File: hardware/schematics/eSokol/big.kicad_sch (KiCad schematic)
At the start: 34 parts, among them J6 BIGBATT_CHRG, M1 MY1016Z2, M2 FAN1, Q10 AO3401A, Q11 BC547, Q12 S8550, Q13 BC547, Q14 S8550, Q4 BC547, SW2 SW_MEASURE, SW8 SW_KEY, U10 LB27, U11 DS_VC288, U7 49e, U8 DS18S20

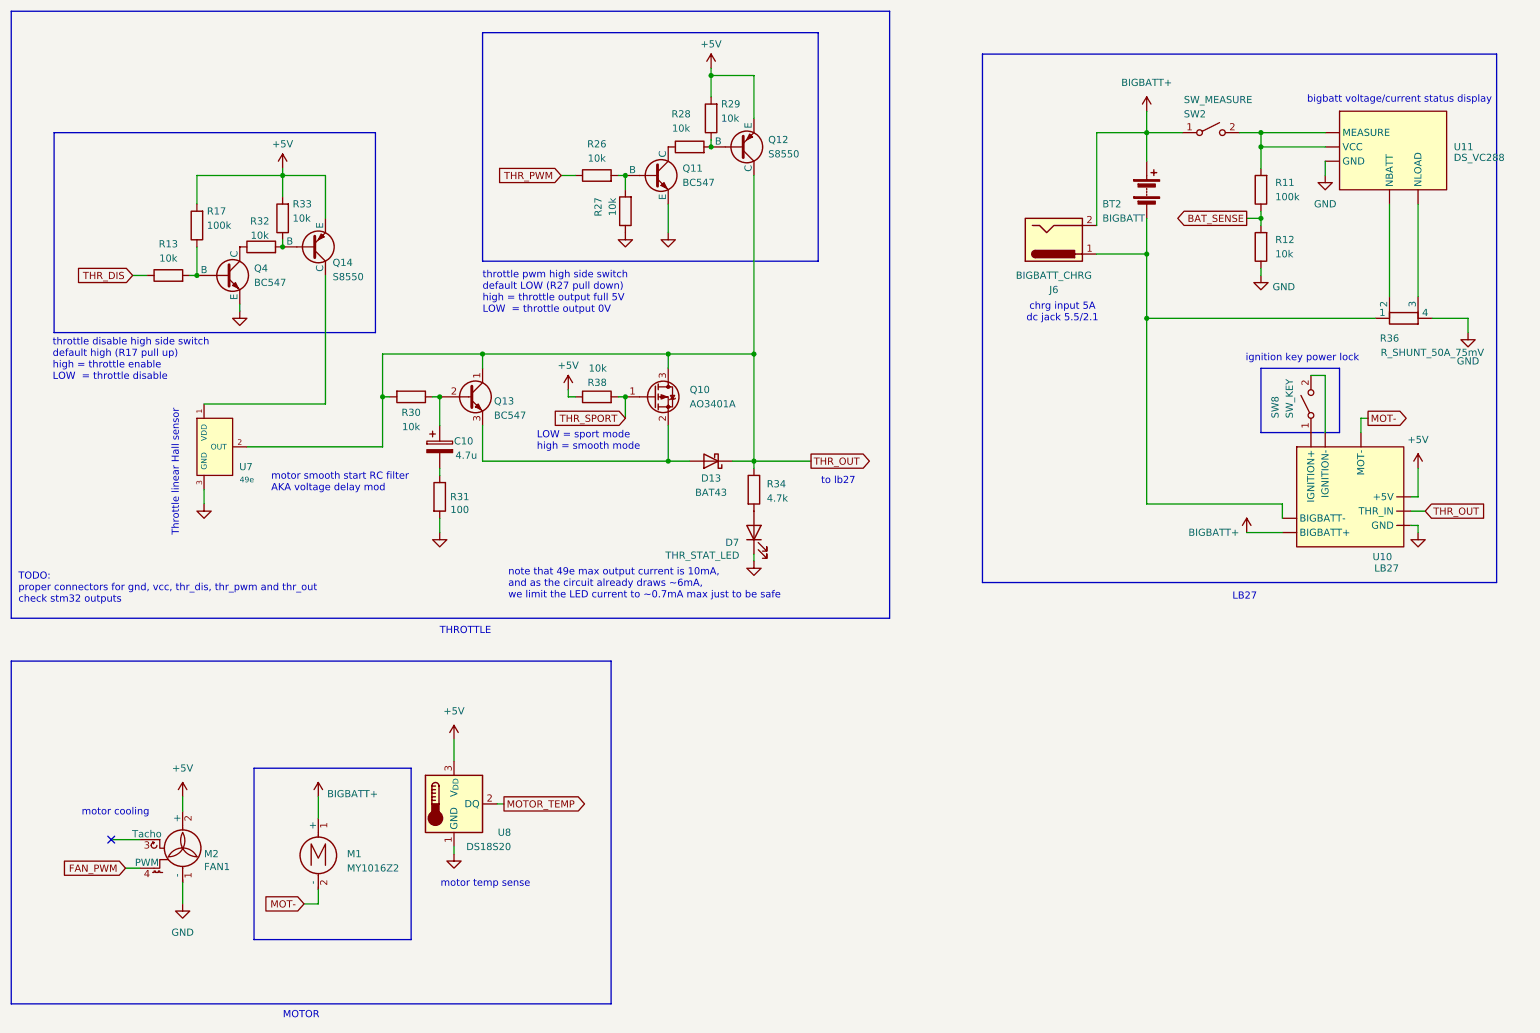
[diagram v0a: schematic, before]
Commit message: WIP: update some schematics to reflect the newest design changes
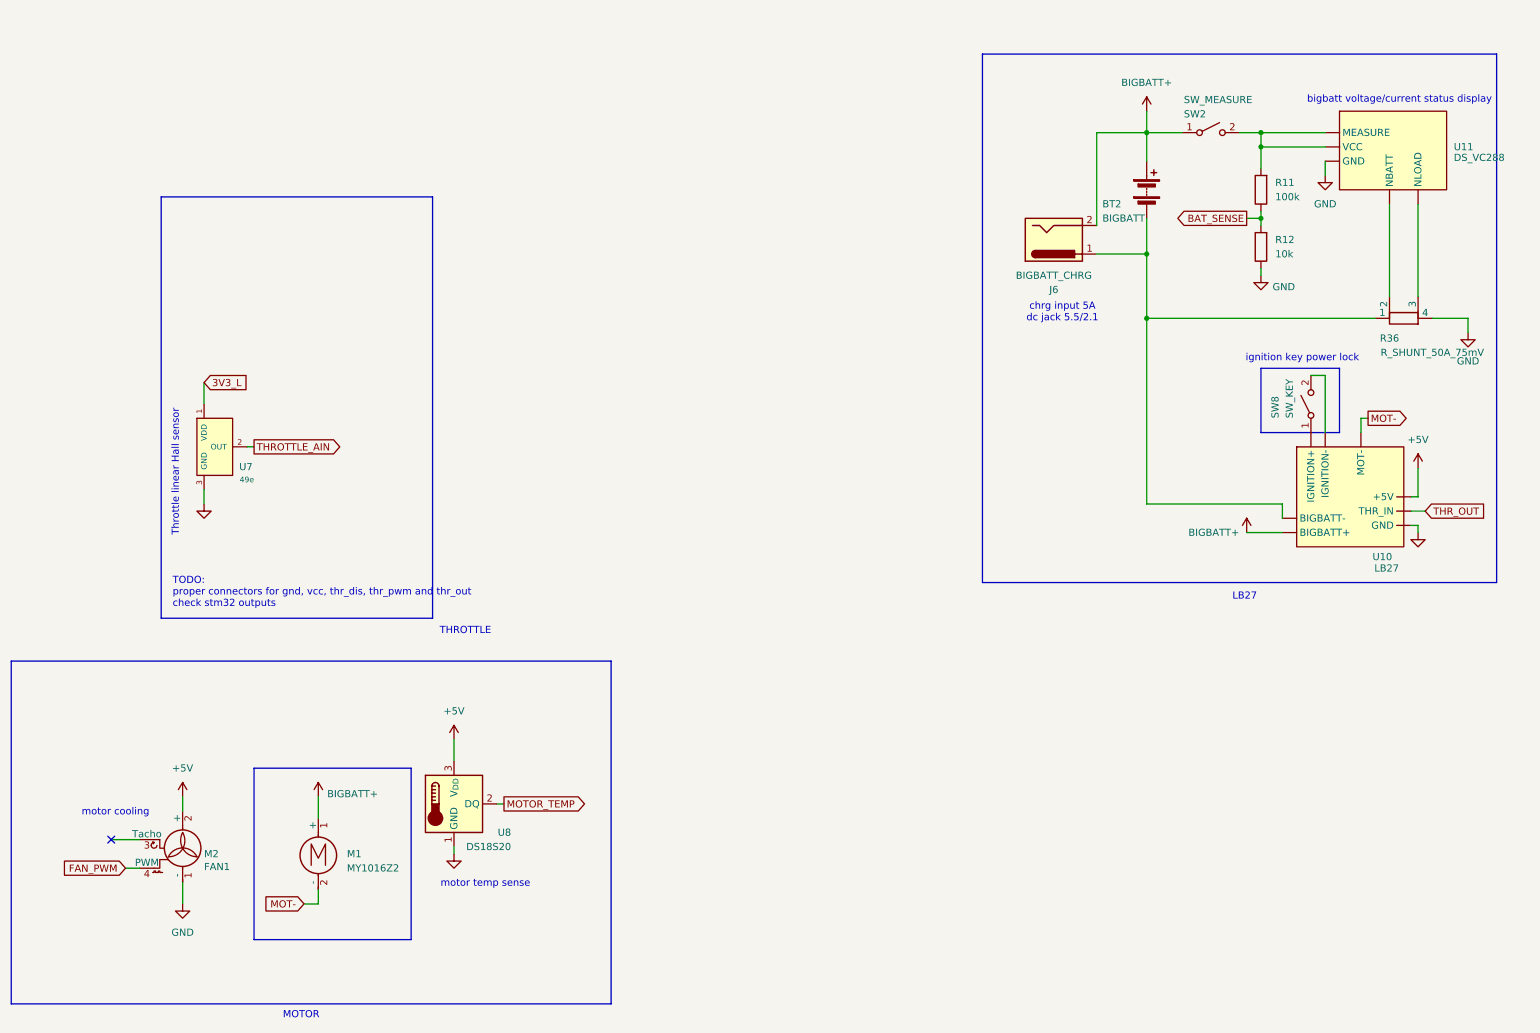
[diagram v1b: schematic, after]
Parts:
- removed C10: 4.7u, symbol Device:C_Polarized
- removed D13: BAT43, Diode_THT:D_DO-35_SOD27_P7.62mm_Horizontal, symbol Diode:BAT43
- removed D7: THR_STAT_LED, symbol Device:LED
- removed Q10: AO3401A, Package_TO_SOT_SMD:SOT-23, symbol Transistor_FET:AO3401A
- removed Q11, Q4: BC547, symbol Simulation_SPICE:NPN
- removed Q12, Q14: S8550, symbol Simulation_SPICE:PNP
- removed Q13: BC547, Package_TO_SOT_THT:TO-92_Inline, symbol Transistor_BJT:BC547
- removed R13, R26, R27, R28, R29, R30, R32, R33, R38: 10k, symbol Device:R
- removed R17: 100k, symbol Device:R
- removed R31: 100, symbol Device:R
- removed R34: 4.7k, symbol Device:R
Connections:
- net THR_OUT: no longer U7.2 (OUT)
- net 3V3_L: now reaches U7.1 (VDD)
- new net THROTTLE_AIN: U7.2 (OUT)
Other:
- note removed: "LOW = sport mode high = smooth mode"
- note removed: "motor smooth start RC filter AKA voltage delay mod"
- note removed: "note that 49e max output current is 10mA, and as the circuit already draws ~6mA, we limit the LED current to ~0.7mA max just to be safe"
- note removed: "throttle disable high side switch default high (R17 pull up) high = throttle enable LOW = throttle disable"
- note removed: "throttle pwm high side switch default LOW (R27 pull down) high = throttle output full 5V LOW = throttle output 0V"
- note removed: "to lb27"
